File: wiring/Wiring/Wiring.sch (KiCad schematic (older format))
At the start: 4 parts

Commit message: Add layout
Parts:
- U1, U2, U3, U4: renamed from U?; footprint (none) -> Package_DFN_QFN:DFN-8-1EP_4x4mm_P0.8mm_EP2.5x3.6mm
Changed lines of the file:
@@
 $EndDescr
 $Comp
-L Wiring:F U?
+L Wiring:F U3
 U 1 1 5ED38158
 P 7050 5850
-F 0 "U?" H 7678 5929 50  0001 L CNN
+F 0 "U3" H 7678 5929 50  0001 L CNN
 F 1 "F" H 7650 5450 50  0000 L CNN
-F 2 "" H 7000 6000 50  0001 C CNN
+F 2 "Package_DFN_QFN:DFN-8-1EP_4x4mm_P0.8mm_EP2.5x3.6mm" H 7000 6000 50  0001 C CNN
 F 3 "" H 7000 6000 50  0001 C CNN
 	1    7050 5850
@@
 $EndComp
 $Comp
-L Wiring:E U?
+L Wiring:E U2
 U 1 1 5ED38C33
 P 5200 2550
-F 0 "U?" H 4525 3500 50  0001 C CNN
+F 0 "U2" H 4525 3500 50  0001 C CNN
 F 1 "E" H 4550 1700 50  0000 C CNN
-F 2 "" H 5200 2550 50  0001 C CNN
+F 2 "Package_DFN_QFN:DFN-8-1EP_4x4mm_P0.8mm_EP2.5x3.6mm" H 5200 2550 50  0001 C CNN
 F 3 "" H 5200 2550 50  0001 C CNN
 	1    5200 2550
@@
 $EndComp
 $Comp
-L Wiring:G U?
+L Wiring:G U4
 U 1 1 5ED3C88F
 P 7200 1150
-F 0 "U?" H 7378 1196 50  0001 L CNN
+F 0 "U4" H 7378 1196 50  0001 L CNN
 F 1 "G" H 7050 1000 50  0000 L CNN
-F 2 "" H 7200 1150 50  0001 C CNN
+F 2 "Package_DFN_QFN:DFN-8-1EP_4x4mm_P0.8mm_EP2.5x3.6mm" H 7200 1150 50  0001 C CNN
 F 3 "" H 7200 1150 50  0001 C CNN
 	1    7200 1150
@@
 	7250 750  7250 850
 $Comp
-L Wiring:MAIN U?
+L Wiring:MAIN U1
 U 1 1 5ED3FA8D
 P 4650 5700
-F 0 "U?" H 3600 5850 50  0001 L CNN
+F 0 "U1" H 3600 5850 50  0001 L CNN
 F 1 "MAIN" H 5550 5550 50  0000 L CNN
-F 2 "" H 4650 6000 50  0001 C CNN
+F 2 "Package_DFN_QFN:DFN-8-1EP_4x4mm_P0.8mm_EP2.5x3.6mm" H 4650 6000 50  0001 C CNN
 F 3 "" H 4650 6000 50  0001 C CNN
 	1    4650 5700

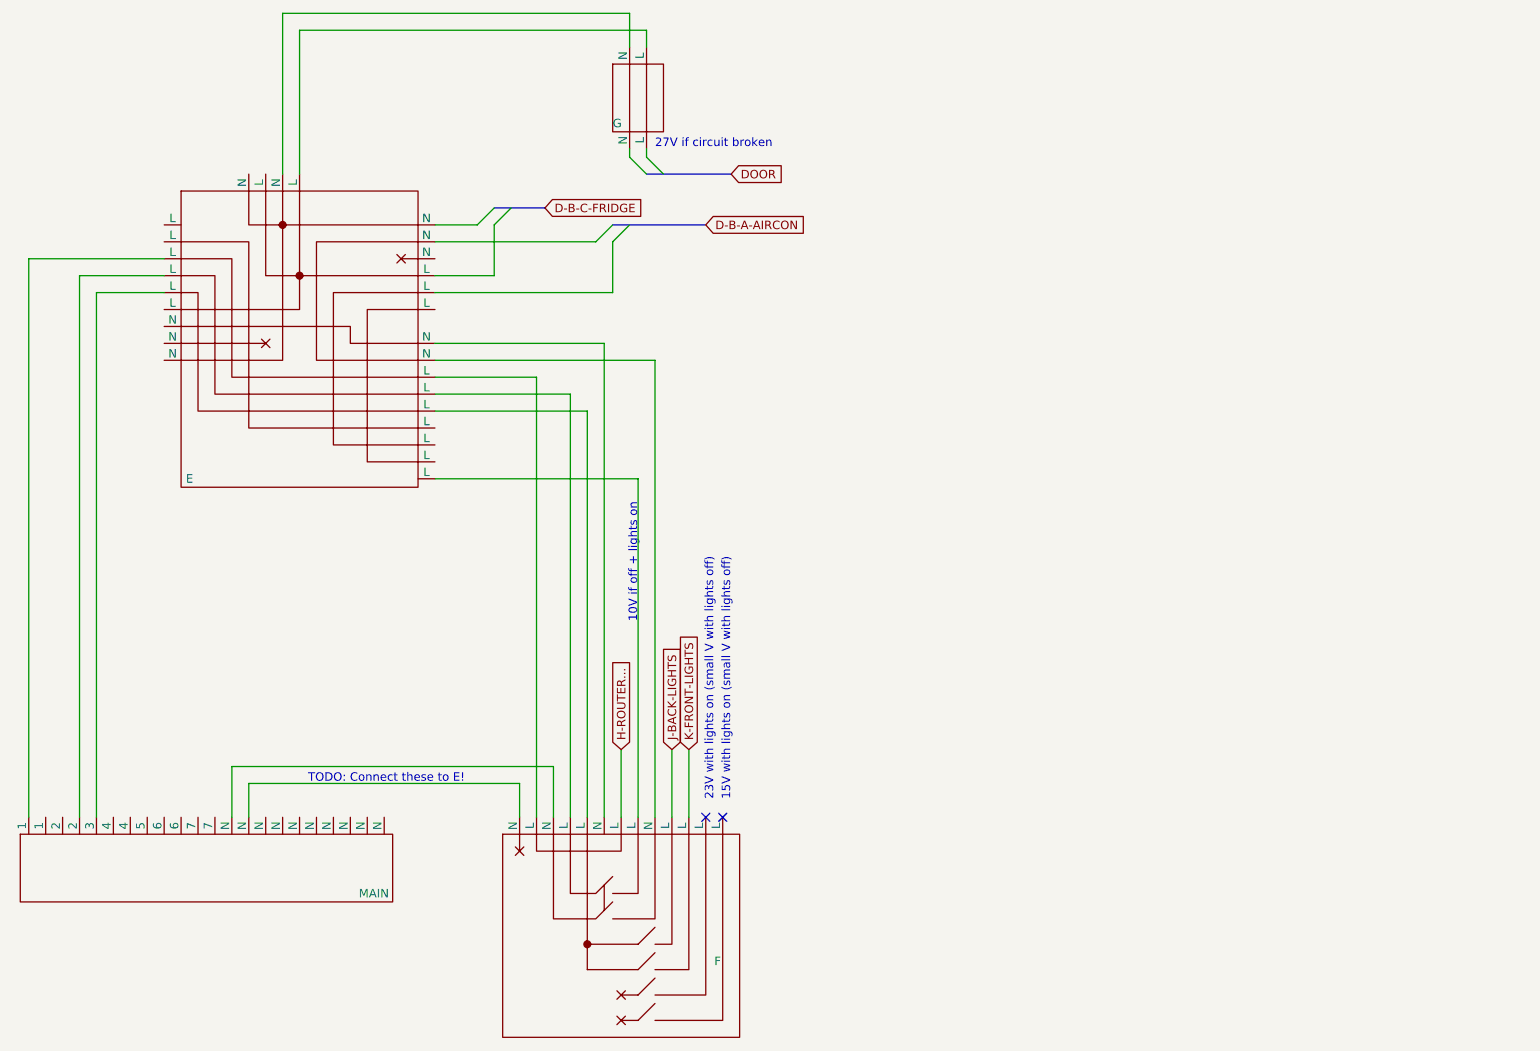
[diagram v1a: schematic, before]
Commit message: Add rough outlines of boxes H, I, J
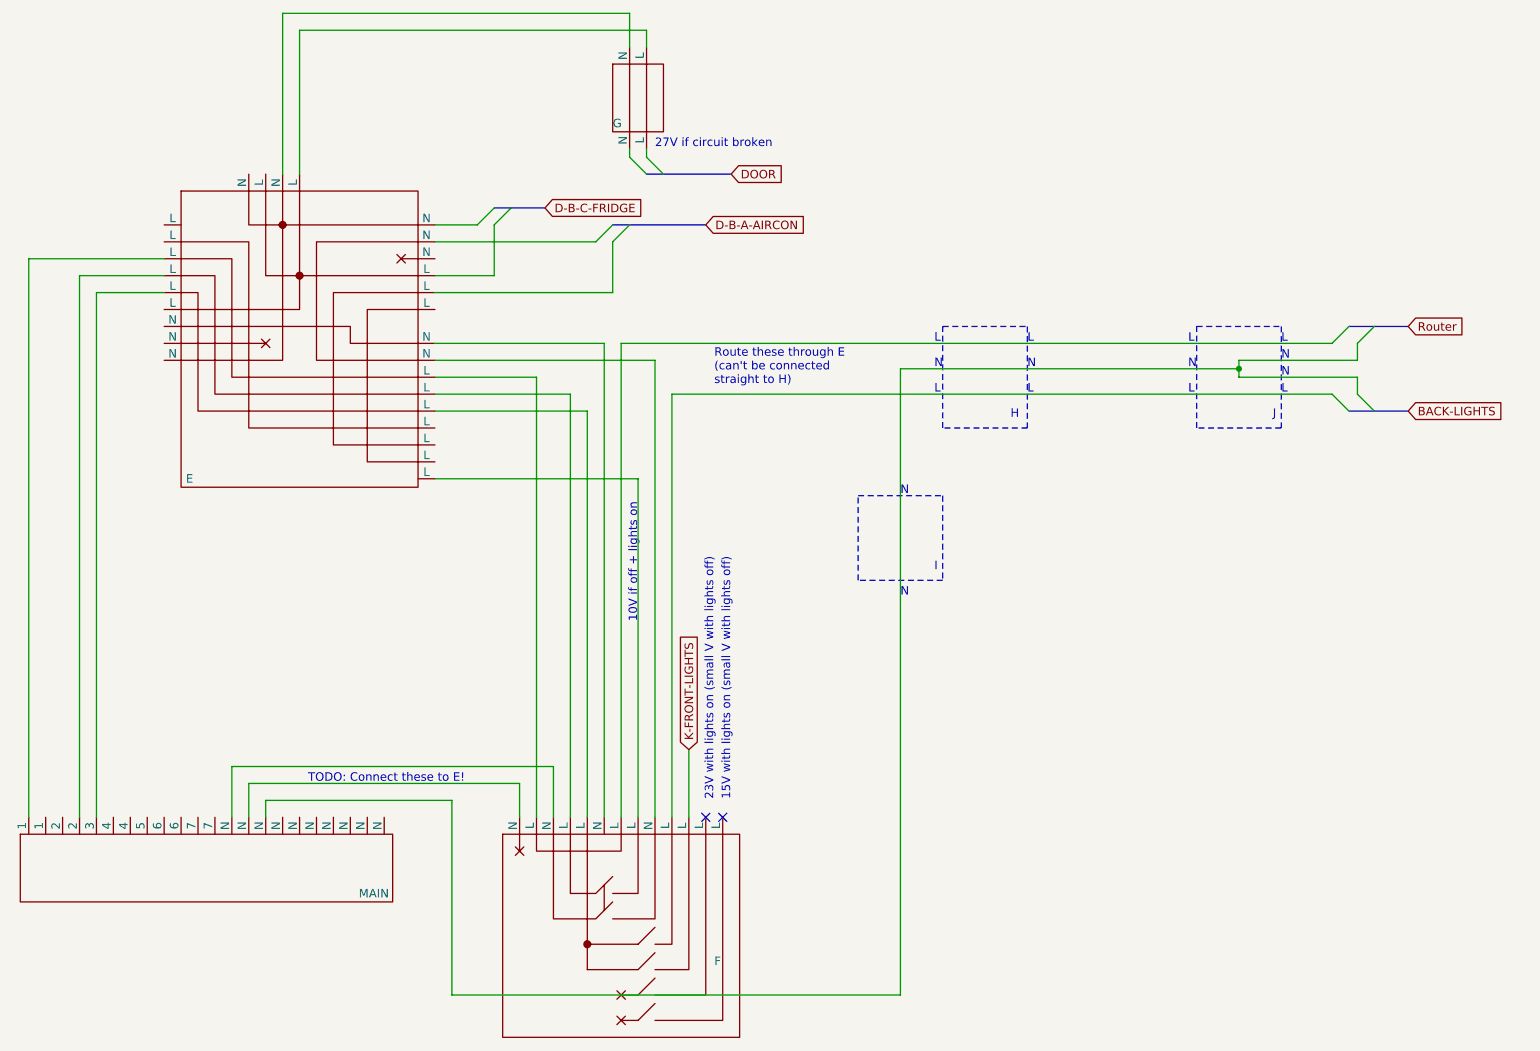
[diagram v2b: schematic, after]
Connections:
- net H-ROUTER...: no longer names the net of U3.7 (L)
- net J-BACK-LIGHTS: no longer names the net of U3.10 (L)
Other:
- note added: "H"
- note added: "I"
- note added: "J"
- note added: "L"
- note added: "N"
- note added: "Route these through E\n(can't be connected \nstraight to H)"
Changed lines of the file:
@@
 D-B-C-FRIDGE
-Wire Wire Line
-	7100 5000 7100 5400
-Text GLabel 7100 5000 1    50   Input ~ 0
-H-ROUTER...
-Text GLabel 7400 5000 1    50   Input ~ 0
-J-BACK-LIGHTS
-Wire Wire Line
-	7400 5000 7400 5400
 Wire Wire Line
 	6700 5400 6700 5100
@@
 Wire Wire Line
 	6000 3000 6900 3000
-Wire Bus Line
-	6350 1800 6650 1800
-Wire Bus Line
-	7250 1600 7750 1600
-Wire Bus Line
-	7050 1900 7600 1900
 Wire Wire Line
 	4000 2300 4000 5400
@@
 Text Notes 7300 1450 0    50   ~ 0
 27V if circuit broken
+Wire Notes Line
+	9000 2500 9500 2500
+Wire Notes Line
+	9500 2500 9500 3100
+Wire Notes Line
+	9000 3100 9000 2500
+Text Notes 9400 3050 0    50   ~ 0
+H
+Wire Notes Line
+	10500 2500 11000 2500
+Wire Notes Line
+	11000 2500 11000 3100
+Wire Notes Line
+	11000 3100 10500 3100
+Wire Notes Line
+	10500 3100 10500 2500
+Text Notes 10950 3050 0    50   ~ 0
+J
+Wire Wire Line
+	7100 2600 7100 5400
+Text GLabel 11750 2500 2    50   Input ~ 0
+Router
+Entry Wire Line
+	11300 2600 11400 2500
+Wire Wire Line
+	11300 2600 7100 2600
+Wire Wire Line
+	5000 5400 5000 5300
+Wire Wire Line
+	5000 5300 6100 5300
+Wire Wire Line
+	6100 5300 6100 6450
+Wire Wire Line
+	6100 6450 8750 6450
+Wire Wire Line
+	8750 6450 8750 2750
+Entry Wire Line
+	11550 2500 11450 2600
+Wire Wire Line
+	11450 2700 11450 2600
+Wire Notes Line
+	8500 3500 9000 3500
+Wire Notes Line
+	9000 3500 9000 4000
+Wire Notes Line
+	9000 4000 8500 4000
+Wire Notes Line
+	8500 4000 8500 3500
+Text Notes 8950 3950 0    50   ~ 0
+I
+Wire Wire Line
+	7400 2900 11300 2900
+Wire Wire Line
+	7400 2900 7400 5400
+Wire Notes Line
+	9500 3100 9000 3100
+Text Notes 7650 2850 0    50   ~ 0
+Route these through E\n(can't be connected \nstraight to H)
+Wire Wire Line
+	10750 2700 11450 2700
+Wire Wire Line
+	10750 2750 10750 2700
+Wire Wire Line
+	8750 2750 10750 2750
+Wire Wire Line
+	10750 2750 10750 2800
+Wire Wire Line
+	10750 2800 11450 2800
+Connection ~ 10750 2750
+Text Notes 11000 2600 0    50   ~ 0
+L
+Text Notes 11000 2700 0    50   ~ 0
+N
+Text Notes 11000 2800 0    50   ~ 0
+N
+Text Notes 11000 2900 0    50   ~ 0
+L
+Text Notes 10450 2600 0    50   ~ 0
+L
+Text Notes 10450 2750 0    50   ~ 0
+N
+Text Notes 10450 2900 0    50   ~ 0
+L
+Text Notes 9500 2600 0    50   ~ 0
+L
+Text Notes 9500 2900 0    50   ~ 0
+L
+Text Notes 9500 2750 0    50   ~ 0
+N
+Text Notes 8950 2750 0    50   ~ 0
+N
+Text Notes 8950 2600 0    50   ~ 0
+L
+Text Notes 8950 2900 0    50   ~ 0
+L
+Text Notes 8750 3500 0    50   ~ 0
+N
+Text Notes 8750 4100 0    50   ~ 0
+N
+Text GLabel 11750 3000 2    50   Input ~ 0
+BACK-LIGHTS
+Entry Wire Line
+	11300 2900 11400 3000
+Entry Wire Line
+	11450 2900 11550 3000
+Wire Wire Line
+	11450 2800 11450 2900
+Wire Bus Line
+	11400 3000 11750 3000
+Wire Bus Line
+	11400 2500 11750 2500
+Wire Bus Line
+	6350 1800 6650 1800
+Wire Bus Line
+	7250 1600 7750 1600
+Wire Bus Line
+	7050 1900 7600 1900
 $EndSCHEMATC
